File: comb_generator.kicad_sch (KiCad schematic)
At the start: 28 parts, among them J2 RFShield_TwoPieces, U1 ISL3280ExHZ, U4 KT2520K-T, U5 Si5351C-B-GM, U6 GALI-5, U7 PAT1220-C-3DB

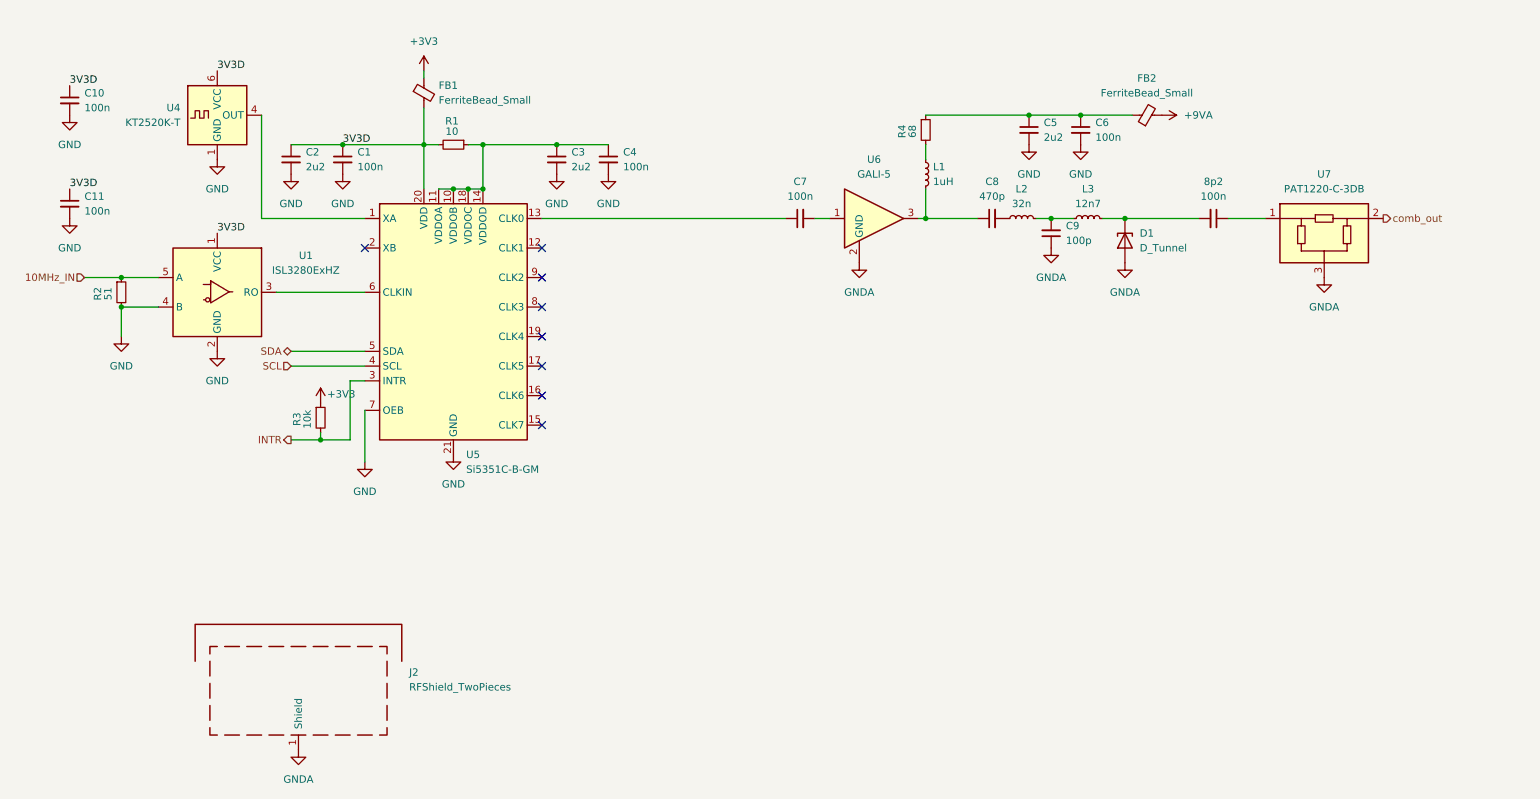
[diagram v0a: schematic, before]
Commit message: weiter layoutet...
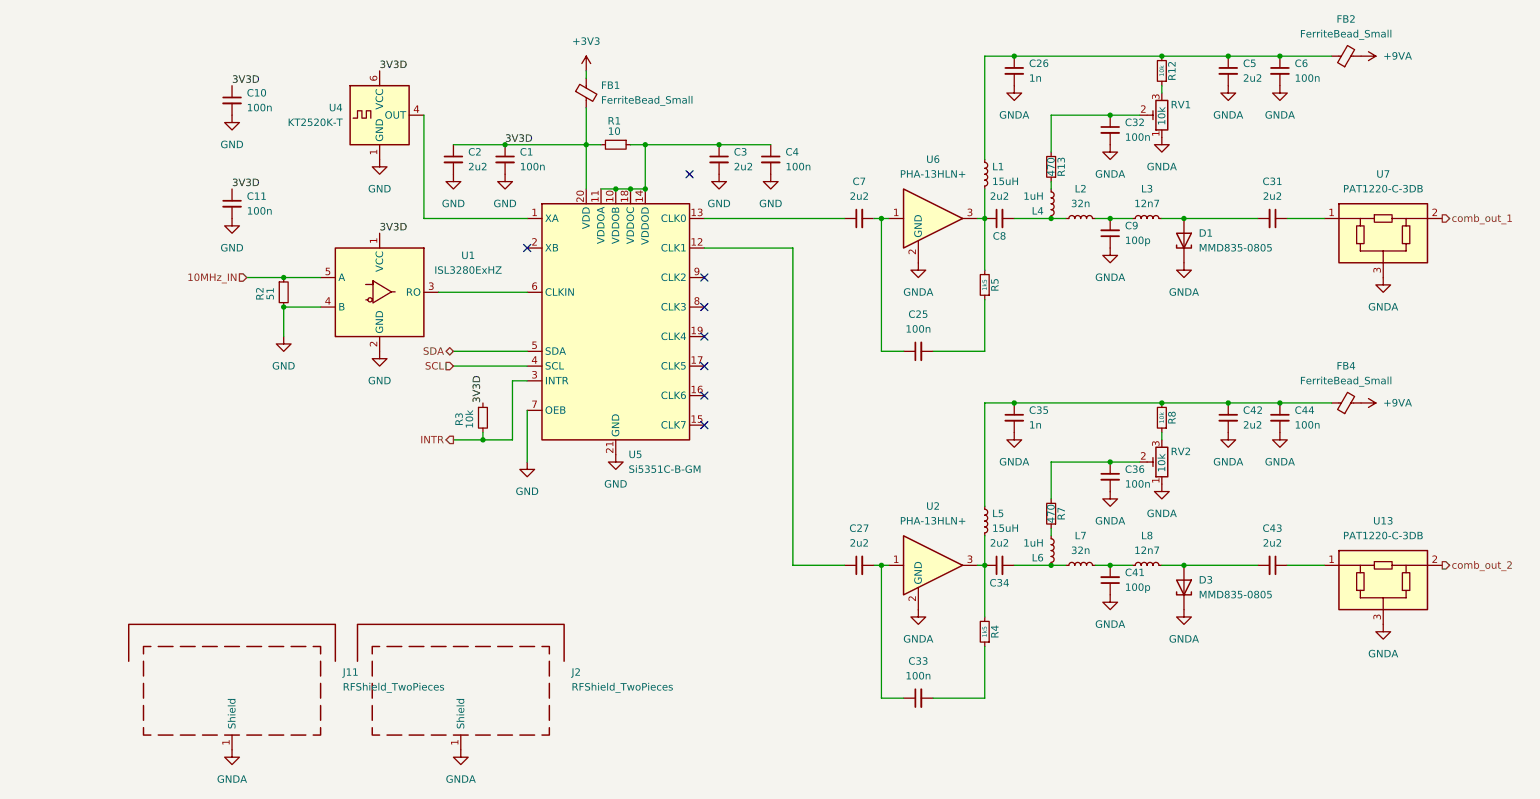
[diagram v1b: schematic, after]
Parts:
- added C25, C32, C33, C36, C44: 100n, Capacitor_SMD:C_0805_2012Metric_Pad1.18x1.45mm_HandSolder, symbol Device:C_Small
- added C26, C35: 1n, Capacitor_SMD:C_0805_2012Metric_Pad1.18x1.45mm_HandSolder, symbol Device:C_Small
- added C27, C34, C42, C43: 2u2, Capacitor_SMD:C_0805_2012Metric_Pad1.18x1.45mm_HandSolder, symbol Device:C_Small
- added C41: 100p, Capacitor_SMD:C_0805_2012Metric_Pad1.18x1.45mm_HandSolder, symbol Device:C_Small
- added D3: MMD835-0805, Diode_SMD:D_0805_2012Metric_Pad1.15x1.40mm_HandSolder, symbol Device:D_Tunnel
- added FB4: FerriteBead_Small, Inductor_SMD:L_0805_2012Metric_Pad1.15x1.40mm_HandSolder, symbol Device:FerriteBead_Small
- added J11: RFShield_TwoPieces, RF_Shielding:Wuerth_36103305_30x30mm, symbol Device:RFShield_TwoPieces
- added L4, L6: 1uH, Inductor_SMD:L_0805_2012Metric_Pad1.05x1.20mm_HandSolder, symbol Device:L_Small
- added L5: 15uH, Inductor_SMD:L_0805_2012Metric_Pad1.05x1.20mm_HandSolder, symbol Device:L_Small
- added L7: 32n, Inductor_SMD:L_0805_2012Metric_Pad1.05x1.20mm_HandSolder, symbol Device:L_Small
- added L8: 12n7, Inductor_SMD:L_0805_2012Metric_Pad1.05x1.20mm_HandSolder, symbol Device:L_Small
- added R12, R8: 10k, Resistor_SMD:R_0805_2012Metric_Pad1.20x1.40mm_HandSolder, symbol Device:R_Small
- added R13, R7: 470, Resistor_SMD:R_0805_2012Metric_Pad1.20x1.40mm_HandSolder, symbol Device:R_Small
- added R5: 1k5, Resistor_SMD:R_0805_2012Metric_Pad1.20x1.40mm_HandSolder, symbol Device:R_Small
- added RV1, RV2: 10k, Potentiometer_SMD:Potentiometer_Bourns_3214J_Horizontal, symbol Device:R_Potentiometer_Trim
- added U13: PAT1220-C-3DB, RF_Converter:RF_Attenuator_Susumu_PAT1220, symbol RF:PAT1220-C-3DB
- added U2: PHA-13HLN+, Package_TO_SOT_SMD:SOT-89-3, symbol RF_Amplifier:GALI-5
- C1, C10, C11, C2, C3, C4, C5, C6, C9: footprint Capacitor_SMD:C_0603_1608Metric_Pad1.08x0.95mm_HandSolder -> Capacitor_SMD:C_0805_2012Metric_Pad1.18x1.45mm_HandSolder
- C31: renamed from 8p2; value 100n -> 2u2; footprint Capacitor_SMD:C_0603_1608Metric_Pad1.08x0.95mm_HandSolder -> Capacitor_SMD:C_0805_2012Metric_Pad1.18x1.45mm_HandSolder
- C7: value 100n -> 2u2; footprint Capacitor_SMD:C_0603_1608Metric_Pad1.08x0.95mm_HandSolder -> Capacitor_SMD:C_0805_2012Metric_Pad1.18x1.45mm_HandSolder
- C8: value 470p -> 2u2; footprint Capacitor_SMD:C_0603_1608Metric_Pad1.08x0.95mm_HandSolder -> Capacitor_SMD:C_0805_2012Metric_Pad1.18x1.45mm_HandSolder
- D1: value D_Tunnel -> MMD835-0805; Distributor (none) -> Mouser; Distributor PN (none) -> 937-MMD835-0805; Manufacturer (none) -> MACOM; Manufacturer PN (none) -> MMD835-0805
- J2: footprint RF_Shielding:Wuerth_36503305_30x30mm -> RF_Shielding:Wuerth_36103305_30x30mm
- L1: value 1uH -> 15uH
- R1, R2, R3: footprint Resistor_SMD:R_0603_1608Metric_Pad0.98x0.95mm_HandSolder -> Resistor_SMD:R_0805_2012Metric_Pad1.20x1.40mm_HandSolder
- R4: value 68 -> 1k5; footprint Resistor_SMD:R_0603_1608Metric_Pad0.98x0.95mm_HandSolder -> Resistor_SMD:R_0805_2012Metric_Pad1.20x1.40mm_HandSolder
- U6: value GALI-5 -> PHA-13HLN+; Distributor (none) -> Mouser; Distributor PN (none) -> 139-PHA-13HLN; Manufacturer PN (none) -> PHA-13HLN+
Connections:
- net +3V3: no longer R3.1
- net +9VA: now also FB4.2
- net 3V3D: now also R3.1
- net GND: no longer C5.2, C6.2
- net GNDA: now also C5.2, C6.2, D1.1 (K), C26.2, C32.2, C35.2, C36.2, C41.1, C42.2, C44.2, D3.1 (K), J11.1 (Shield), RV1.1, RV2.1, U13.3, U2.2 (GND); no longer D1.2 (A)
- net at U5.12 (CLK1): now also C27.1
- net at C7.2, U6.1: now also C25.1
- net at C8.1, L1.2, U6.3: now also R5.2
- net at C31.2, L3.2: now also D1.2 (A); no longer D1.1 (K)
- net at C8.2, L2.1: now also L4.2
- net at C5.1, C6.1, FB2.1: now also L1.1, C26.1, R12.2; no longer R4.1
- net at R4.2: now also C34.1, L5.2, U2.3; no longer L1.1
- net comb_out renamed comb_out_1
- new net: C25.2, R5.1
- new net: C34.2, L6.2, L7.1
- new net: C41.2, L7.2, L8.1
- new net: C36.1, R7.2, RV2.2
- new net: R8.1, RV2.3
- new net: C43.2, D3.2 (A), L8.2
- new net: C35.1, C42.1, C44.1, FB4.1, L5.1, R8.2
- new net: L6.1, R7.1
- new net: C43.1, U13.1
- new net: C32.1, R13.2, RV1.2
- new net: L4.1, R13.1
- new net: C27.2, C33.1, U2.1
- new net: C33.2, R4.1
- new net: R12.1, RV1.3
- new net comb_out_2: U13.2
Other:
- moved on the sheet: C1, C10, C11, C2, C3, C31, C4, C5, C6, C7, C8, C9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

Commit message: es wird langsam...
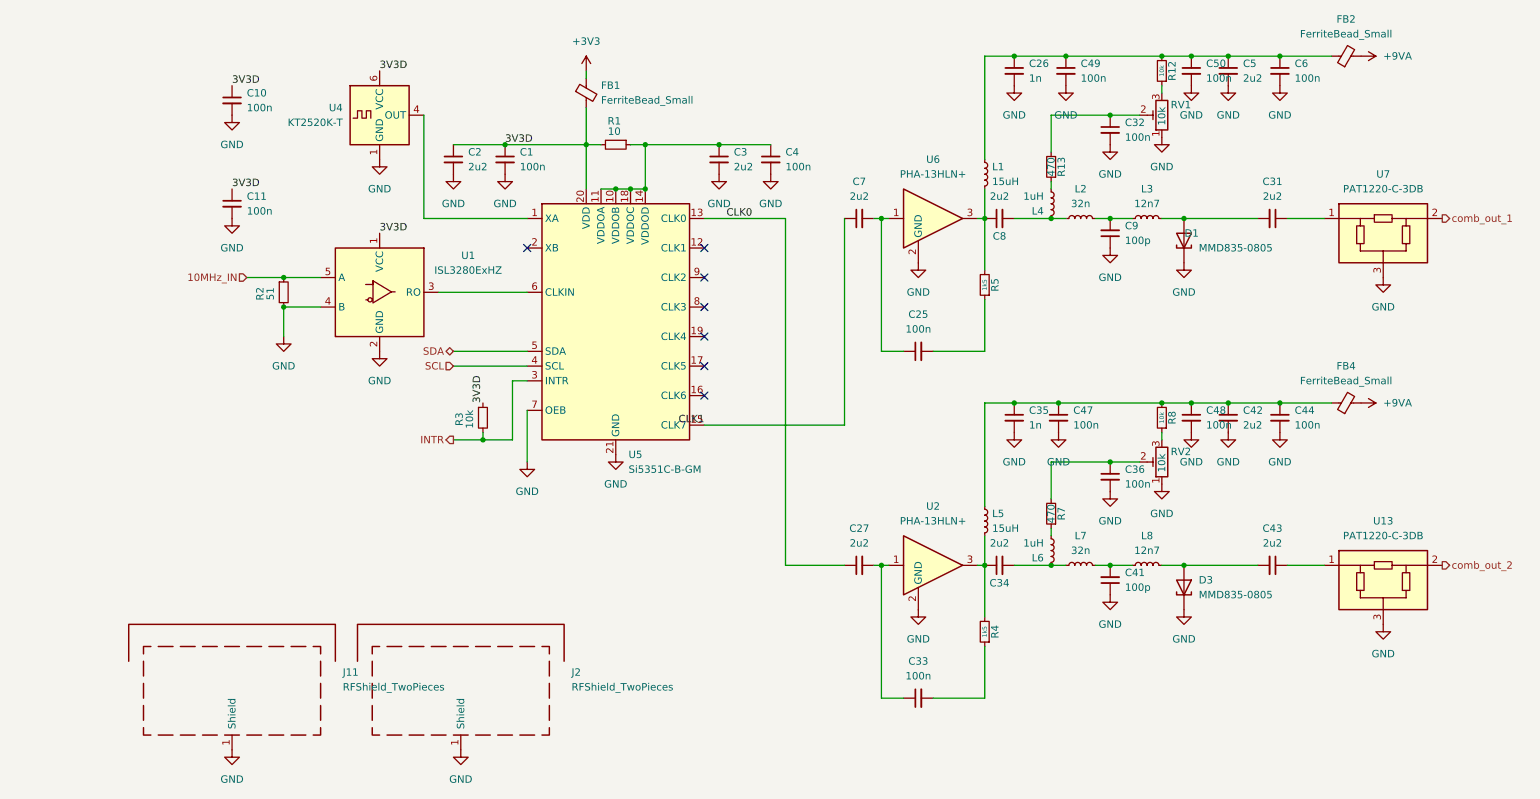
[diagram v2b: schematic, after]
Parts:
- added C47, C48, C49, C50: 100n, Capacitor_SMD:C_0805_2012Metric_Pad1.18x1.45mm_HandSolder, symbol Device:C_Small
- J11, J2: footprint RF_Shielding:Wuerth_36103305_30x30mm -> RF_Shielding:Wuerth_3670473_47.3x23.3
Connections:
- net GNDA is gone; now on net GND: C26.2, C32.2, C35.2, C36.2, C41.1, C42.2, C44.2, C5.2, C6.2, C9.1, D1.1 (K), D3.1 (K), J11.1 (Shield), J2.1 (Shield), RV1.1, RV2.1, U13.3, U2.2 (GND), U6.2 (GND), U7.3
- net GND: now also C47.2, C48.2, C49.2, C50.2
- net at U5.12 (CLK1): no longer C27.1
- net CLK0: now reaches U5.13 (CLK0)
- net CLK0: now also C27.1; no longer C7.1
- net CLK1: now reaches U5.15 (CLK7)
- net CLK1: now also C7.1
- net at C35.1, C42.1, C44.1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: now also C47.1, C48.1
- net at C26.1, C5.1, C6.1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: now also C49.1, C50.1
- no-connect marks 8 -> 7

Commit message: BOM angefangen und im Layout vom Hundertsten ins Tausendste gekommen...
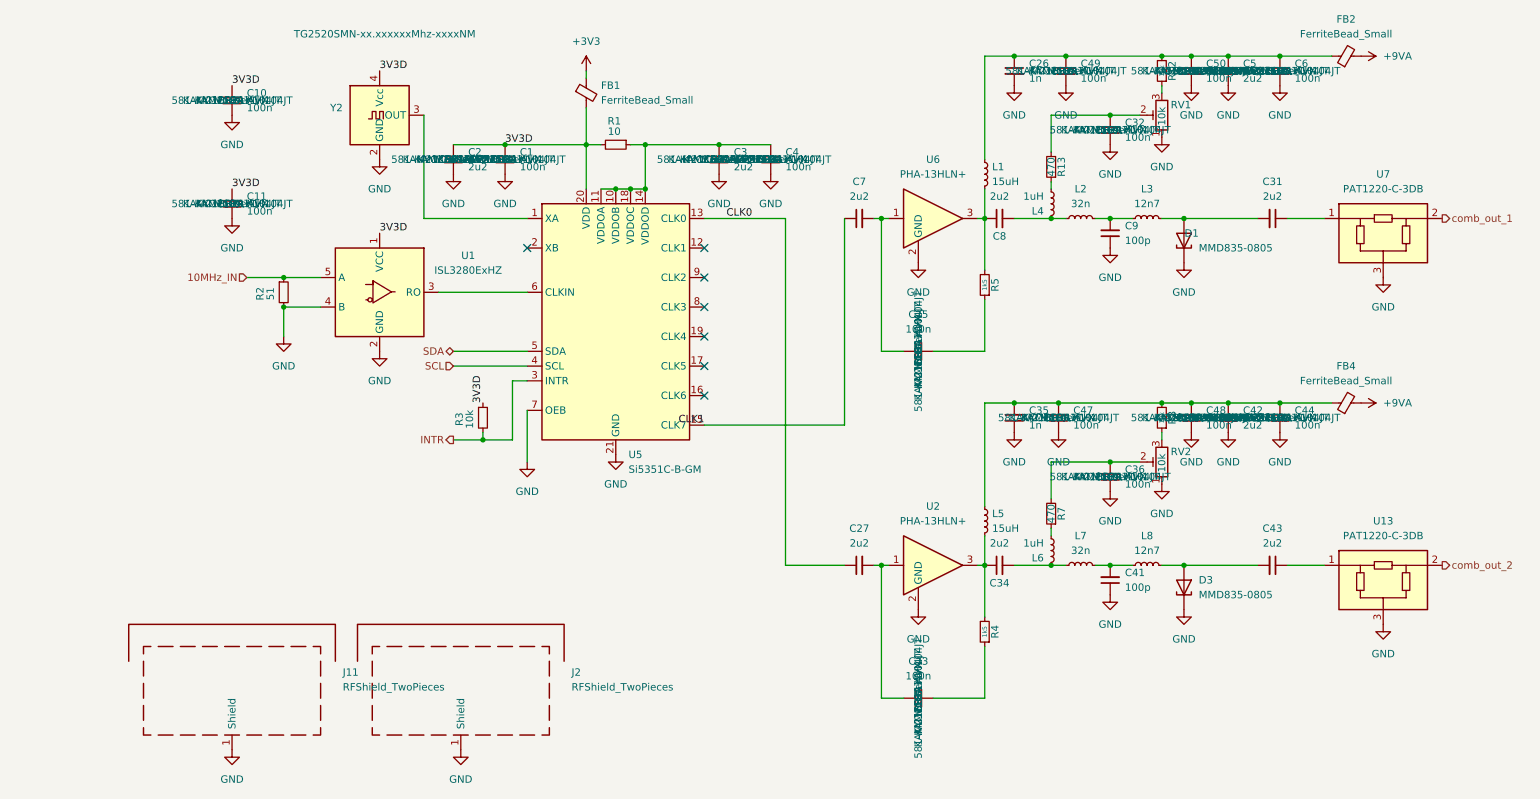
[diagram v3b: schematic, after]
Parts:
- removed U4: KT2520K-T, Oscillator:Oscillator_SMD_Kyocera_2520-6Pin_2.5x2.0mm, symbol Oscillator:KT2520K-T
- added Y2: TG2520SMN-xx.xxxxxxMhz-xxxxNM, Oscillator:Oscillator_SMD_SeikoEpson_TG2520SMN-xxx-xxxxxx-4Pin_2.5x2.0mm, symbol Oscillator:TG2520SMN-xx.xxxxxxMhz-xxxxNM
- C1, C10, C11, C25, C32, C33, C36, C4, C44, C47, C48, C49, C50, C6: Distributor (none) -> Mouser; Distributor PN (none) -> 581-KAM21BR71H104JT; Manufacturer (none) -> KYOCERA AVX; Manufacturer PN (none) -> KAM21BR71H104JT
- C2, C27, C3, C31, C34, C42, C43, C5, C7, C8: Distributor (none) -> Mouser; Distributor PN (none) -> 581-KAM21KR71E225KU; Manufacturer (none) -> KYOCERA AVX; Manufacturer PN (none) -> KAM21KR71E225KU
- J11, J2: Distributor (none) -> Mouser; Distributor PN (none) -> 710-3670473; Manufacturer (none) -> Wurth Elektronik; Manufacturer PN (none) -> 3670473
- RV1, RV2: footprint Potentiometer_SMD:Potentiometer_Bourns_3214J_Horizontal -> Potentiometer_SMD:Potentiometer_Bourns_TC33X_Vertical
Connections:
- net 3V3D: now also Y2.4 (Vcc)
- net GND: now also Y2.2 (GND)
- net at U5.1 (XA): now also Y2.3 (OUT)
